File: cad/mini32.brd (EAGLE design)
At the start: 66 x 35 mm, 54 parts, among them CN1 MICROSDPLAIN, J1 HEADER-5X1, Q1 MOSFETSOT-23, SW2 SWITCHKMR211, SW3 SWITCHKMR211, U1 STM32F411/48, U2 LSM303D, U3 ADP5062, U4 MCP1824, U5 MAX17048, X1 12MHz, X2 32k768

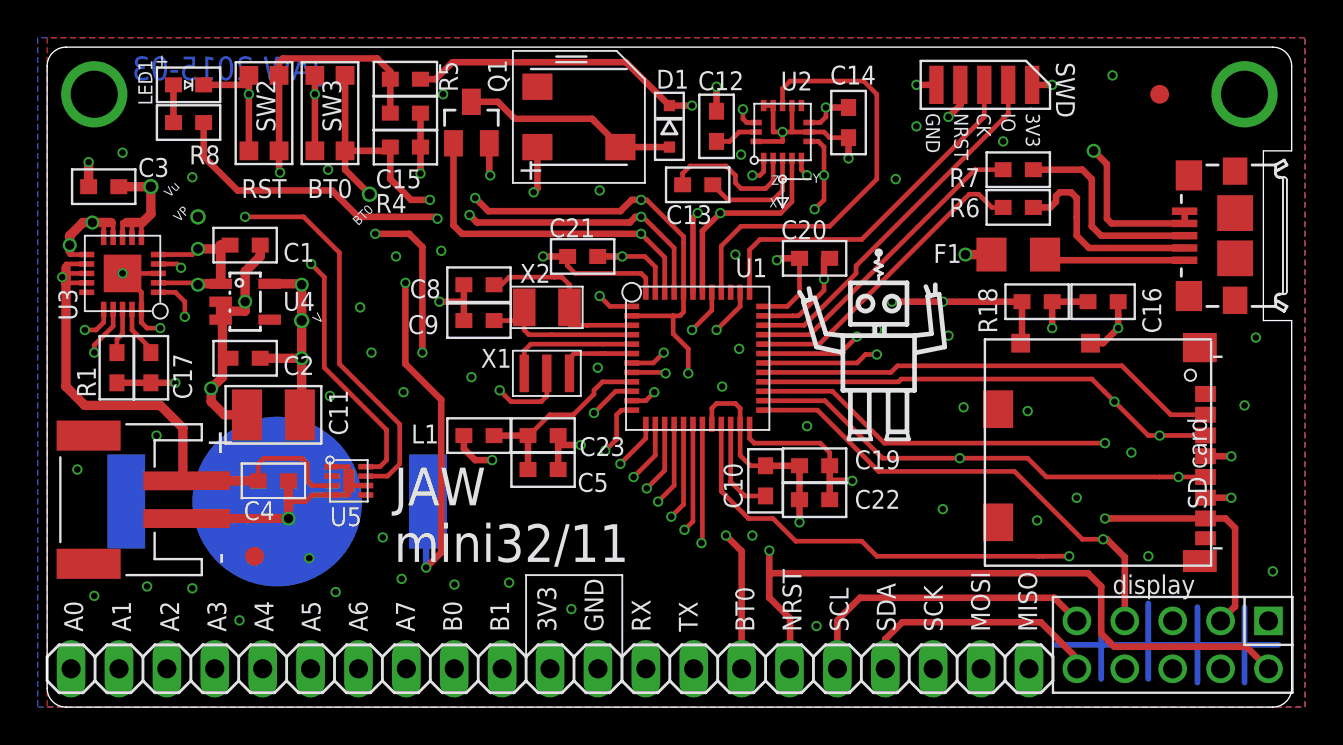
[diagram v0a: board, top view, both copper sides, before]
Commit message: tweak
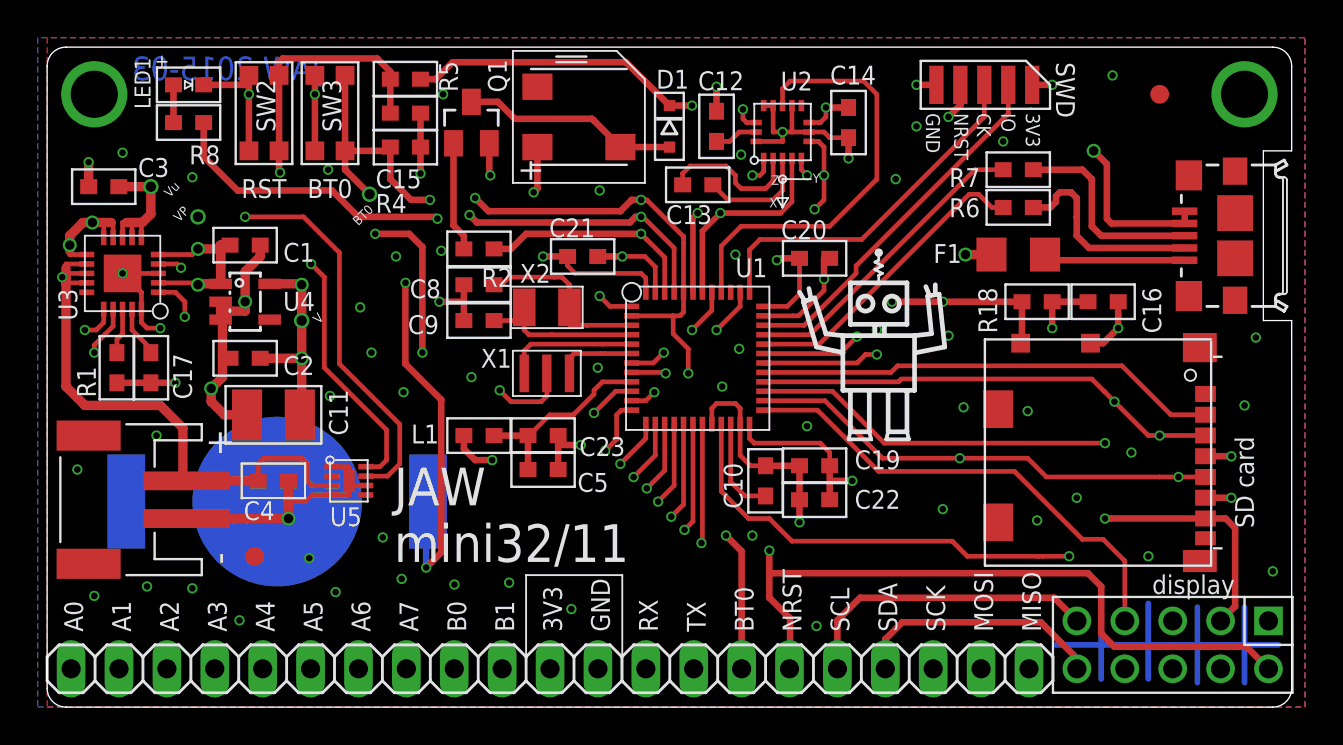
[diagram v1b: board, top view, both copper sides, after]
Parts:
- added R2: 100, jaw:SMD0603
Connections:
- new net N$9: Q1.1, R2.2
- net IOB9: now also R2.1; no longer Q1.1
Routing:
- net IOB9: track 18.1 -> 11.7 mm
- net N$9: track 0.00 -> 5.83 mm
- net DPYCS: track 25.8 -> 25.6 mm, vias 1 -> 0
